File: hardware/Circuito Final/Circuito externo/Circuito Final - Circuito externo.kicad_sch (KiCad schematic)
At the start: 38 parts, among them J1 Conn_02x19_Odd_Even, J2 Conn_02x19_Odd_Even, J3 Conn_01x02, J4 Conn_01x02, SW1 SW_SPDT, SW2 SW_DIP_x04, SW3 SW_DIP_x04, SW4 SW_DIP_x01, SW5 SW_DIP_x01, SW6 SW_DIP_x01, U1 Opamp_Quad, U2 ICL7660

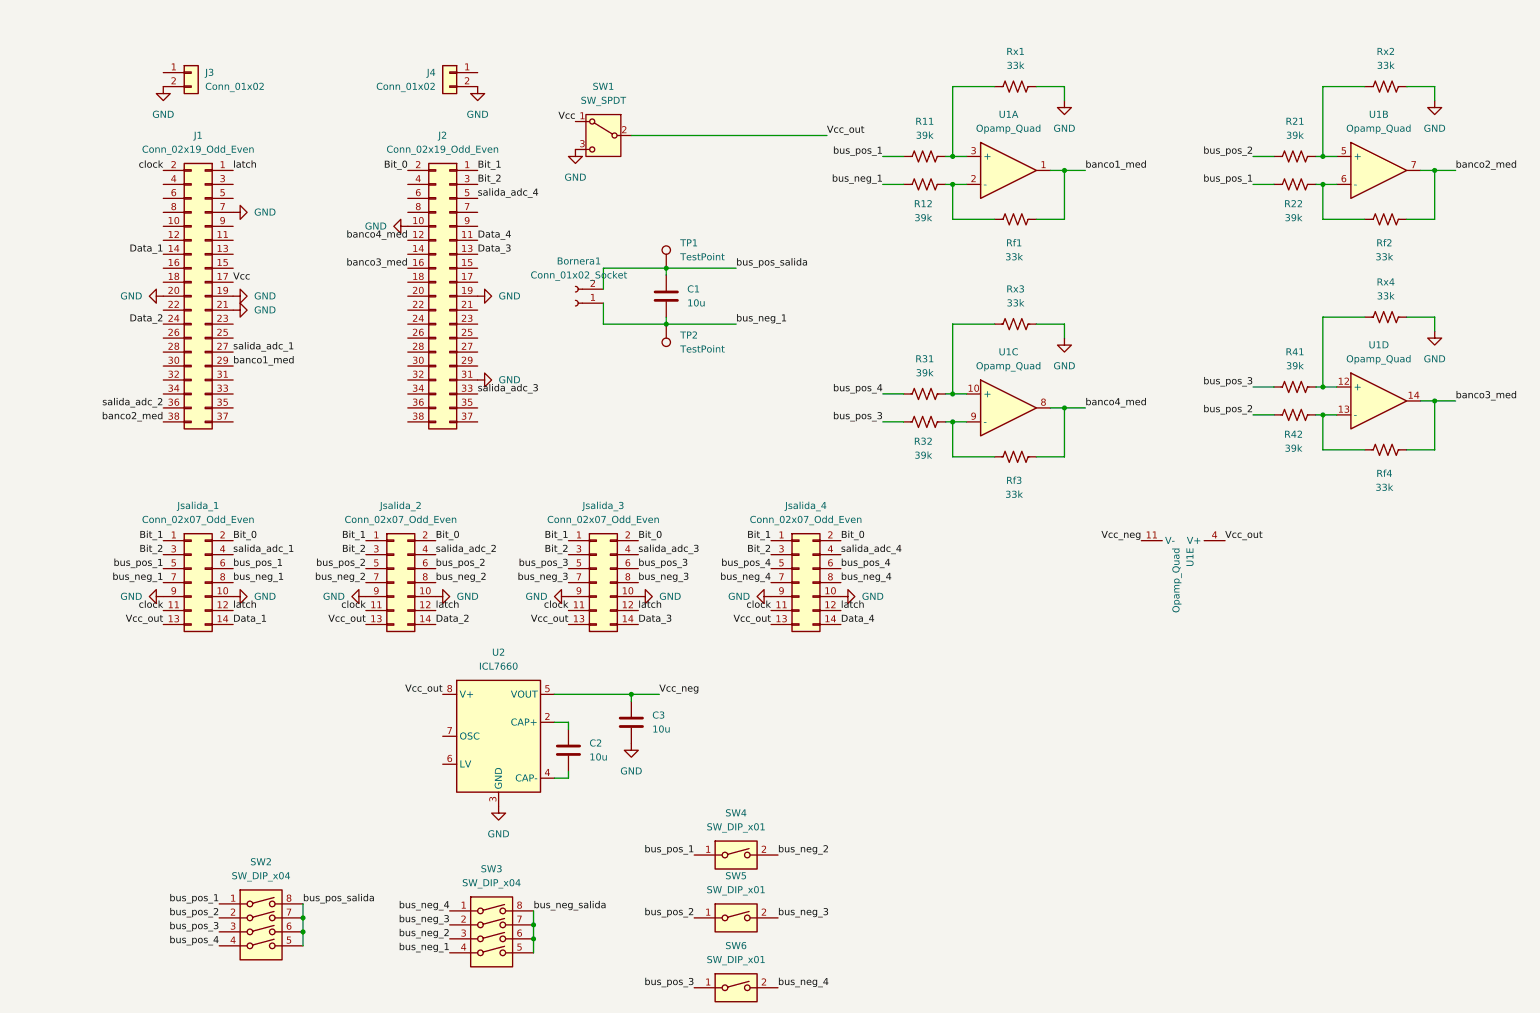
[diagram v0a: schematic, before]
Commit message: sube mediciones y comienza devuelta el conexionado del pcb
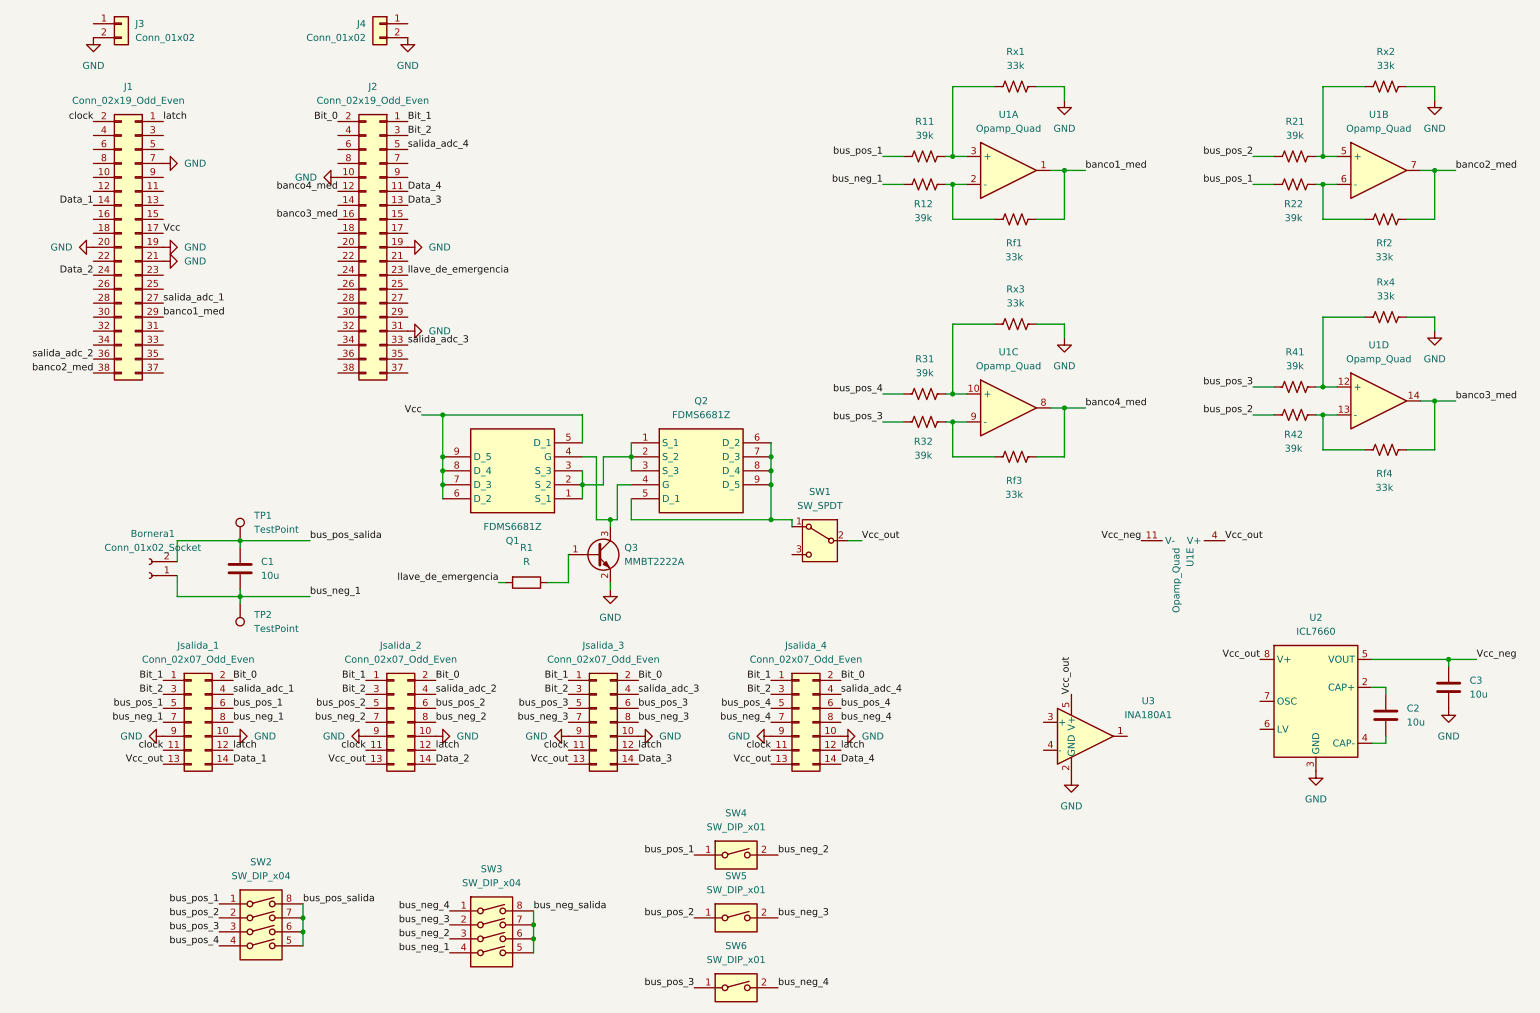
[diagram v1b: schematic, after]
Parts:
- added Q1, Q2: FDMS6681Z, FDMS6681Z, symbol FDMS6681Z:FDMS6681Z
- added Q3: MMBT2222A, Package_TO_SOT_SMD:SOT-23, symbol Transistor_BJT:MMBT2222A
- added R1: R, symbol Device:R
- added U3: INA180A1, Package_TO_SOT_SMD:SOT-23-5, symbol Amplifier_Current:INA180A1
- SW2, SW3: footprint Button_Switch_THT:SW_DIP_SPSTx04_Slide_9.78x12.34mm_W7.62mm_P2.54mm -> Button_Switch_THT:SW_DIP_SPSTx04_Slide_6.7x11.72mm_W7.62mm_P2.54mm_LowProfile
- SW4, SW5, SW6: footprint Button_Switch_THT:SW_DIP_SPSTx01_Slide_6.7x4.1mm_W7.62mm_P2.54mm_LowProfile -> Button_Switch_THT:SW_DIP_SPSTx01_Slide_9.78x4.72mm_W7.62mm_P2.54mm
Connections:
- net GND: now also Q3.2 (E), U3.2 (GND); no longer SW1.3 (C)
- net Vcc: now also Q1.5 (D_1), Q1.6 (D_2), Q1.7 (D_3), Q1.8 (D_4), Q1.9 (D_5); no longer SW1.1 (A)
- net Vcc_out: now also U3.5 (V+)
- net llave_de_emergencia: now reaches J2.23 (Pin_23)
- net llave_de_emergencia: now also R1.2
- new net: Q3.1 (B), R1.1
- new net: Q1.4 (G), Q2.4 (G), Q3.3 (C)
- new net: Q1.1 (S_1), Q1.2 (S_2), Q1.3 (S_3), Q2.1 (S_1), Q2.2 (S_2), Q2.3 (S_3)
- new net: Q2.5 (D_1), Q2.6 (D_2), Q2.7 (D_3), Q2.8 (D_4), Q2.9 (D_5), SW1.1 (A)
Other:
- moved on the sheet: Bornera1, C1, C2, C3, J1, J2, J3, J4, Jsalida_1, Jsalida_2, Jsalida_3, Jsalida_4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
